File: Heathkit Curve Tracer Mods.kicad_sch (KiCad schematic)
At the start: 14 parts, among them J1 Switch, J2 IC6 Jumper, Q1 2N3904, U1 74LS42, U2 74LS90, U3 LM7805_TO220

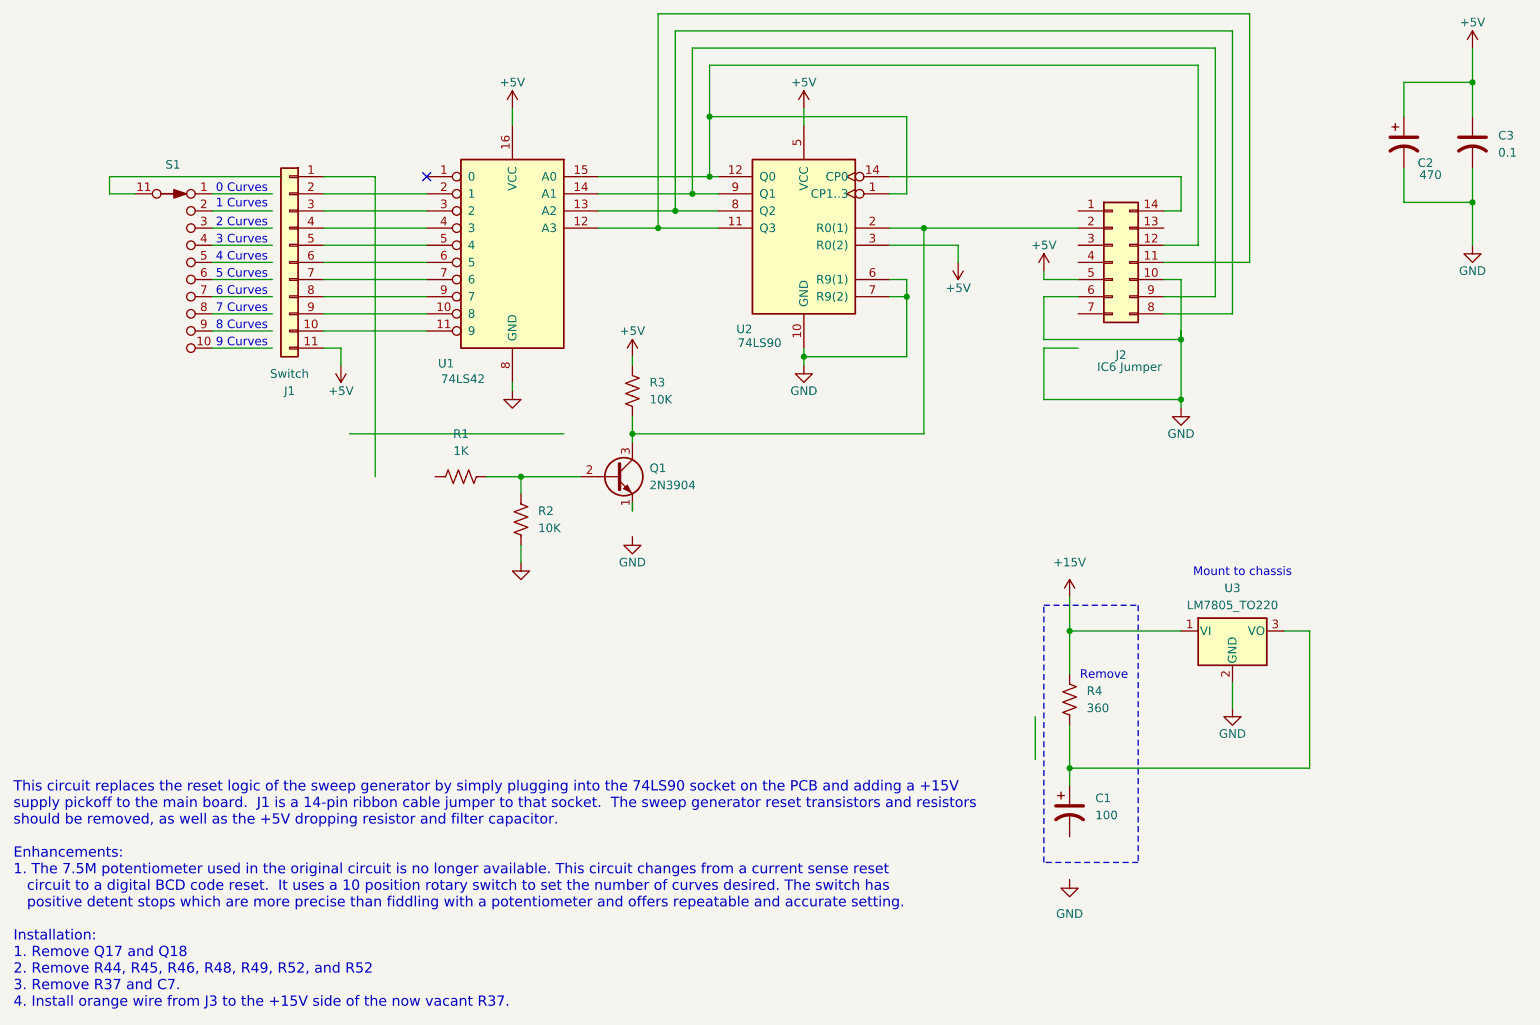
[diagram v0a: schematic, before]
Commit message: Refined traces
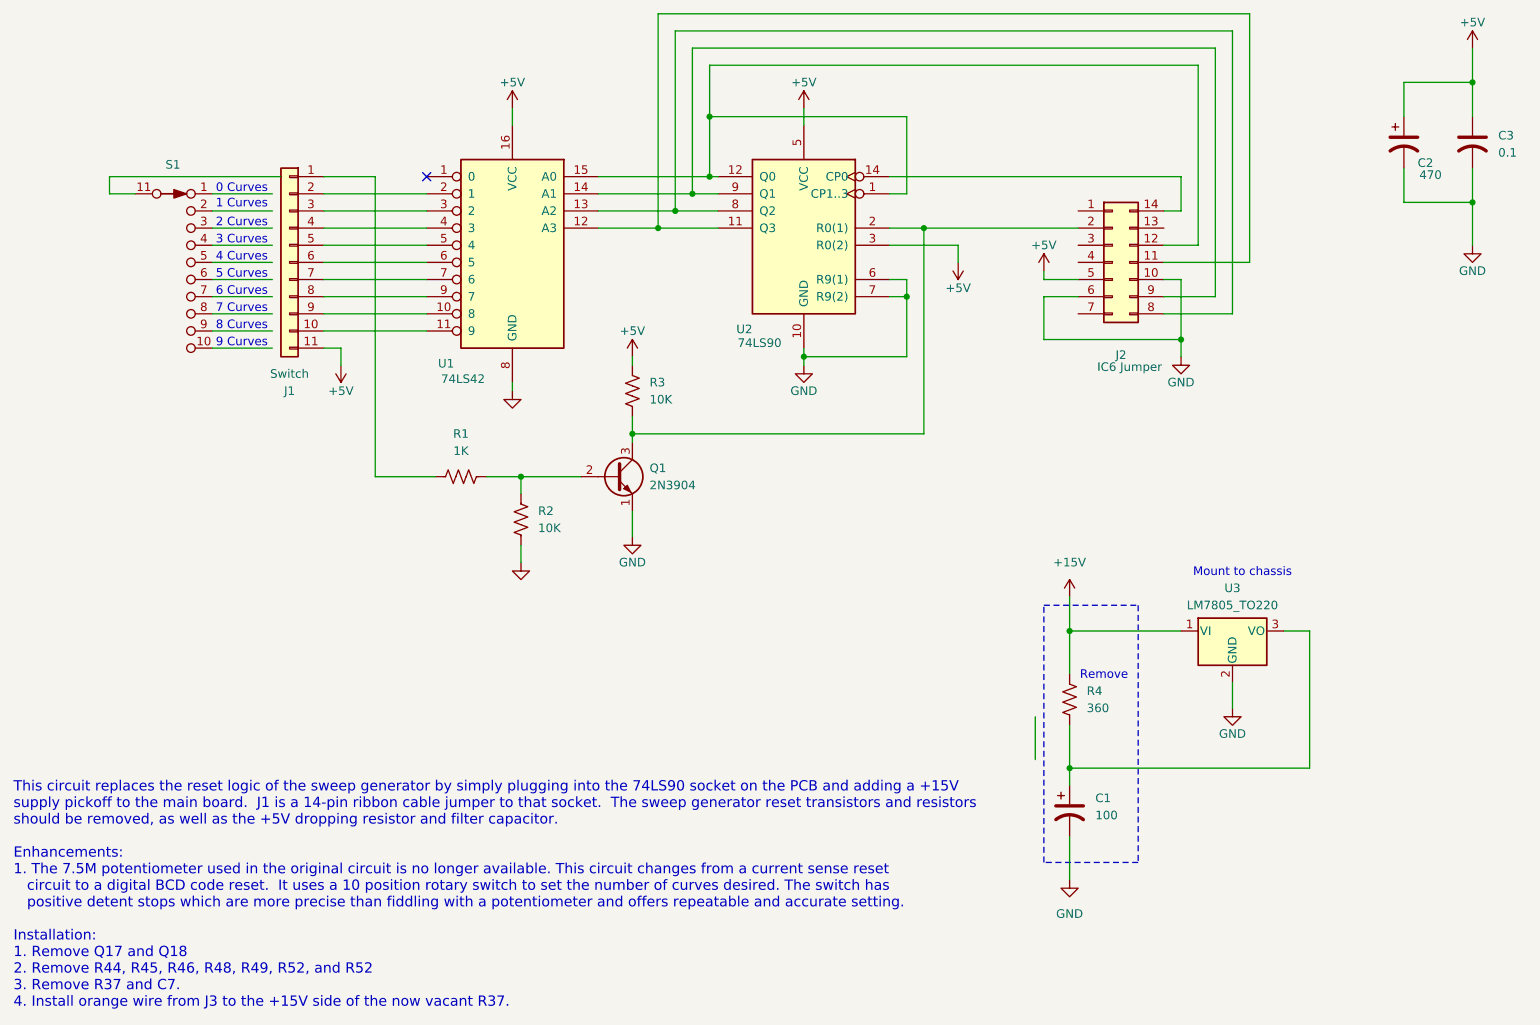
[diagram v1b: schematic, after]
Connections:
- net GND: now also C1.2, Q1.1 (E)
- net at R1.1: now also J1.1 (Pin_1)
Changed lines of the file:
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@@
-	)
-	(junction
-		(at 198.12 85.09)
-		(diameter 0)
-		(color 0 0 0 0)
 	)
 	(junction
@@
 	(wire
 		(pts
+			(xy 181.61 149.86) (xy 181.61 156.21)
+		)
+		(stroke
+			(width 0)
+			(type default)
+		)
+	)
+	(wire
+		(pts
 			(xy 241.3 55.88) (xy 231.14 55.88)
 		)
@@
 	(wire
 		(pts
+			(xy 78.74 96.52) (xy 87.63 96.52)
+		)
+		(stroke
+			(width 0)
+			(type default)
+		)
+	)
+	(wire
+		(pts
 			(xy 128.27 43.18) (xy 128.27 52.07)
 		)
@@
 	(wire
 		(pts
+			(xy 116.84 101.6) (xy 116.84 105.41)
+		)
+		(stroke
+			(width 0)
+			(type default)
+		)
+	)
+	(wire
+		(pts
 			(xy 39.37 54.61) (xy 39.37 52.07)
 		)
@@
 	(wire
 		(pts
-			(xy 198.12 76.2) (xy 198.12 67.31)
-		)
-		(stroke
-			(width 0)
-			(type default)
-		)
-	)
-	(wire
-		(pts
 			(xy 111.76 57.15) (xy 123.19 57.15)
 		)
@@
 	(wire
 		(pts
-			(xy 198.12 86.36) (xy 198.12 85.09)
+			(xy 198.12 67.31) (xy 198.12 78.74)
 		)
 		(stroke
@@
 	(wire
 		(pts
-			(xy 198.12 85.09) (xy 198.12 74.93)
-		)
-		(stroke
-			(width 0)
-			(type default)
-		)
-	)
-	(wire
-		(pts
 			(xy 241.3 43.18) (xy 241.3 38.1)
 		)
@@
 	(wire
 		(pts
-			(xy 177.8 85.09) (xy 198.12 85.09)
-		)
-		(stroke
-			(width 0)
-			(type default)
-		)
-	)
-	(wire
-		(pts
 			(xy 176.53 132.08) (xy 176.53 138.43)
 		)
@@
 	(wire
 		(pts
-			(xy 177.8 77.47) (xy 177.8 85.09)
-		)
-		(stroke
-			(width 0)
-			(type default)
-		)
-	)
-	(wire
-		(pts
-			(xy 74.93 90.17) (xy 106.68 90.17)
-		)
-		(stroke
-			(width 0)
-			(type default)
-		)
-	)
-	(wire
-		(pts
 			(xy 182.88 69.85) (xy 177.8 69.85)
 		)
@@
 		(pts
 			(xy 157.48 43.18) (xy 128.27 43.18)
-		)
-		(stroke
-			(width 0)
-			(type default)
-		)
-	)
-	(wire
-		(pts
-			(xy 182.88 77.47) (xy 177.8 77.47)
-		)
-		(stroke
-			(width 0)
-			(type default)
-		)
-	)
-	(wire
-		(pts
-			(xy 116.84 100.33) (xy 116.84 101.6)
 		)
 		(stroke
@@
 	(symbol
 		(lib_id "power:GND")
-		(at 198.12 86.36 0)
+		(at 198.12 78.74 0)
 		(unit 1)
 		(body_style 1)
@@
 		(dnp no)
 		(property "Reference" "#PWR013"
-			(at 198.12 92.71 0)
+			(at 198.12 85.09 0)
 			(hide yes)
 			(show_name no)
@@
 		)
 		(property "Value" "GND"
-			(at 198.12 90.17 0)
+			(at 198.12 82.55 0)
 			(show_name no)
 			(do_not_autoplace no)
@@
 		)
 		(property "Footprint" ""
-			(at 198.12 86.36 0)
+			(at 198.12 78.74 0)
 			(hide yes)
 			(show_name no)
@@
 		)
 		(property "Datasheet" ""
-			(at 198.12 86.36 0)
+			(at 198.12 78.74 0)
 			(hide yes)
 			(show_name no)
@@
 		)
 		(property "Description" "Power symbol creates a global label with name \"GND\" , ground"
-			(at 198.12 86.36 0)
-			(hide yes)
-			(show_name no)
+			(at 198.12 78.74 0)
+			(hide yes)
+			(show_name no)
